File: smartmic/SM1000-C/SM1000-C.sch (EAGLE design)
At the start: 175 parts, among them CN1 HDR100-3, CN10 MJ-3523-SMT, CN11 HDR100-3, CN12 DF11-16DS, CN2 MOLEX-MINI-B-SMT, CN3 RASM712PX, CN4 RJ-45, CN5 MJ-3523-SMT, CN6 MJ-3523-SMT, CN7 MJ-3523-SMT, CN8 MJ-3523-SMT, CN9 MJ-3523-SMT, J1 JMP-2PIN, J3 JMP-2PIN, J4 JMP-2PIN, J5 JMP-2PIN, P1 TPAD50, P10 TPAD50, P11 TPAD50, P12 TPAD50, P13 TPAD50, P14 TPAD50, P15 TPAD50, P16 TPAD50, P17 TPAD50, P18 TPAD50, P19 TPAD50, P2 TPAD50, P20 TPAD50, P3 TPAD50, P4 TPAD50, P5 TPAD50, P6 TPAD50, P7 TPAD50, P8 TPAD50, P9 TPAD50, SW1 SW-BOURNS-7914S, SW2 SW-BOURNS-7914S, SW3 DPDT, SW4 SW-BOURNS-7914S, T1 SM-LP-5001, T2 SM-LP-5001, U1 STM32F405, U2 LD3985M33R, U3 STMPS2141, U4 EMIF02-USB03F2, U5 TPS54329E, U6 LMV341, U7 LMV341, U8 LM386M-1, U9 LMV341

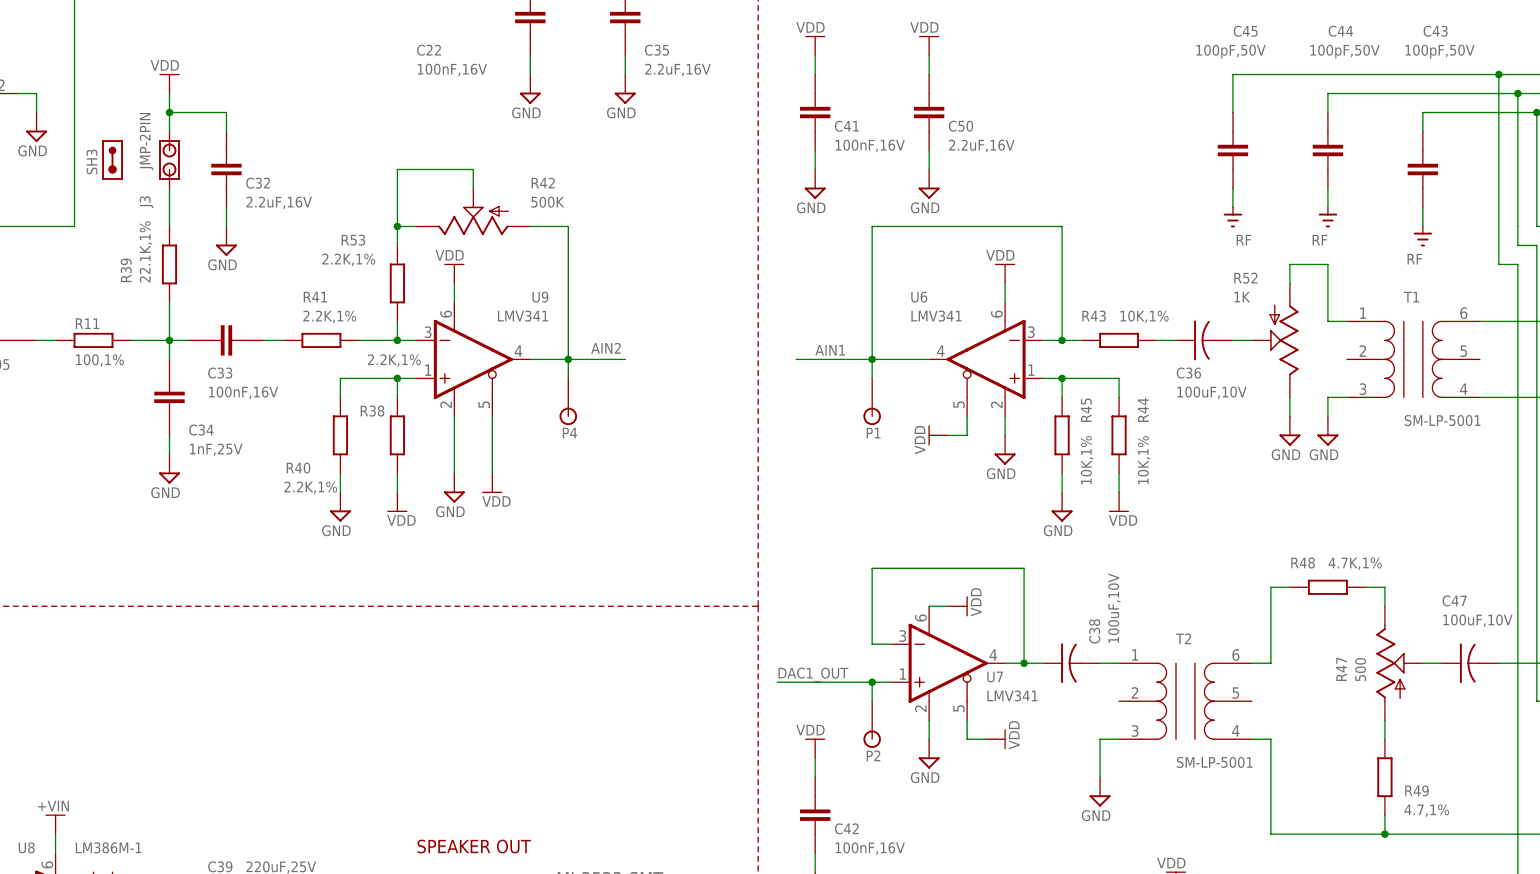
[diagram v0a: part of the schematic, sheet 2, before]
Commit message: Update to reflect review of Change-Log-C.txt  RGB 09/08/2014
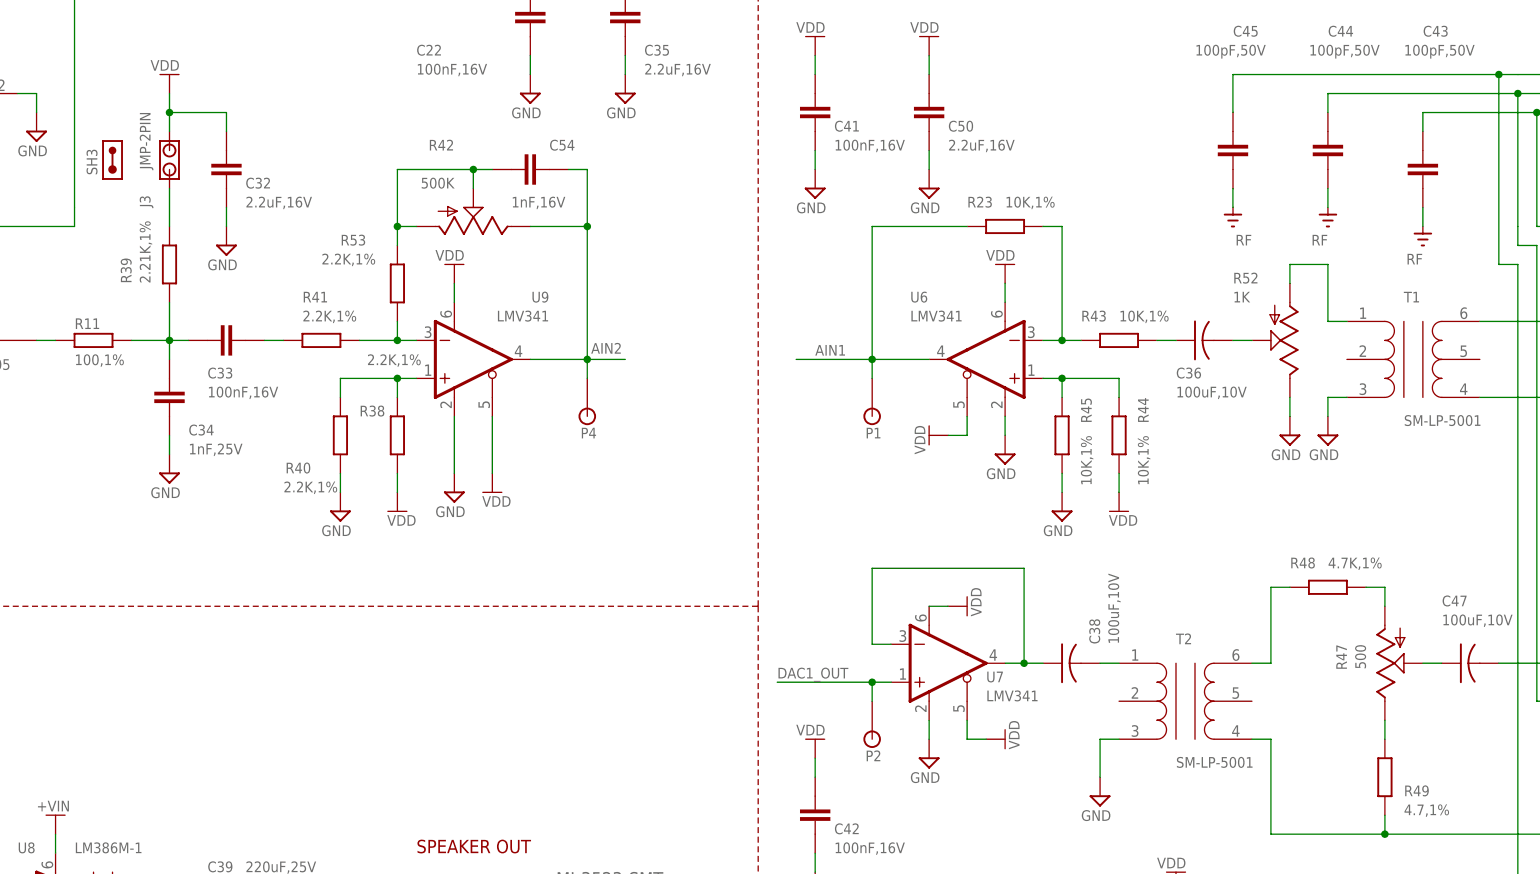
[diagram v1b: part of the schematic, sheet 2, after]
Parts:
- added C54: 1nF,16V, AA-ipc-7351-capacitor:CAPACITOR_0603
- added R23: 10K,1%, AA-ipc-7351-resistor:RESISTOR_0603
- R39: value 22.1K,1% -> 2.21K,1%
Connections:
- removed net N$81: R47.3, R49.2
- new net N$13: R47.1, R49.2
- new net N$14: R23.2, R43.1, U6.-IN
- net AIN1: now also R23.1; no longer R43.1, U6.-IN
- net AIN2: now also C54.2, R42.1; no longer R42.3
- net N$41: now also C54.1, R42.3; no longer R42.1
- net N$82: now also R47.3; no longer R47.1
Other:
- moved on the sheet: P4, R47
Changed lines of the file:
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@@
 <part name="V56" library="A-SUPPLY2" deviceset="GND" device=""/>
 <part name="C34" library="AA-ipc-7351-capacitor" deviceset="CAPACITOR_" device="0603" value="1nF,25V"/>
-<part name="R39" library="AA-ipc-7351-resistor" deviceset="RESISTOR_" device="0603" value="22.1K,1%"/>
+<part name="R39" library="AA-ipc-7351-resistor" deviceset="RESISTOR_" device="0603" value="2.21K,1%"/>
 <part name="R40" library="AA-ipc-7351-resistor" deviceset="RESISTOR_" device="0603" value="2.2K,1%"/>
 <part name="V59" library="A-SUPPLY2" deviceset="GND" device=""/>
@@
 <part name="R22" library="AA-ipc-7351-resistor" deviceset="RESISTOR_" device="0603" value="22.1K,1%"/>
 <part name="V125" library="A-SUPPLY2" deviceset="GND" device=""/>
+<part name="C54" library="AA-ipc-7351-capacitor" deviceset="CAPACITOR_" device="0603" value="1nF,16V"/>
+<part name="R23" library="AA-ipc-7351-resistor" deviceset="RESISTOR_" device="0603" value="10K,1%"/>
 </parts>
 <sheets>
@@
 </instance>
 <instance part="B-FRAME3" gate="G$3" x="355.6" y="279.4" smashed="yes"/>
-<instance part="R47" gate="G$1" x="238.76" y="88.9" smashed="yes">
-<attribute name="NAME" x="233.68" y="86.36" size="1.4224" layer="95" ratio="9" rot="R90"/>
-<attribute name="VALUE" x="236.22" y="86.36" size="1.4224" layer="96" ratio="9" rot="R90"/>
+<instance part="R47" gate="G$1" x="238.76" y="88.9" smashed="yes" rot="MR180">
+<attribute name="NAME" x="233.68" y="91.44" size="1.4224" layer="95" ratio="9" rot="MR270"/>
+<attribute name="VALUE" x="236.22" y="91.44" size="1.4224" layer="96" ratio="9" rot="MR270"/>
 </instance>
 <instance part="R52" gate="G$1" x="226.06" y="132.08" smashed="yes" rot="R180">
@@
 <attribute name="VALUE" x="93.98" y="134.62" size="1.4224" layer="96" ratio="9"/>
 </instance>
-<instance part="R42" gate="G$1" x="116.84" y="147.32" smashed="yes" rot="R90">
-<attribute name="NAME" x="124.46" y="152.4" size="1.4224" layer="95" ratio="9"/>
-<attribute name="VALUE" x="124.46" y="149.86" size="1.4224" layer="96" ratio="9"/>
+<instance part="R42" gate="G$1" x="116.84" y="147.32" smashed="yes" rot="MR90">
+<attribute name="NAME" x="114.3" y="157.48" size="1.4224" layer="95" ratio="9" rot="MR0"/>
+<attribute name="VALUE" x="114.3" y="152.4" size="1.4224" layer="96" ratio="9" rot="MR0"/>
 </instance>
 <instance part="V62" gate="GND" x="99.06" y="109.22" smashed="yes">
@@
 <instance part="P2" gate="G$1" x="170.18" y="83.82" rot="R180"/>
 <instance part="P3" gate="G$1" x="27.94" y="71.12"/>
-<instance part="P4" gate="G$1" x="129.54" y="127" rot="R180"/>
+<instance part="P4" gate="G$1" x="132.08" y="127" rot="R180"/>
 <instance part="C1" gate="G$1" x="101.6" y="251.46" smashed="yes" rot="R90">
 <attribute name="NAME" x="96.52" y="266.7" size="1.4224" layer="95"/>
@@
 <attribute name="VALUE" x="25.4" y="47.498" size="1.4224" layer="96" ratio="9"/>
 </instance>
+<instance part="C54" gate="G$1" x="124.46" y="154.94" smashed="yes">
+<attribute name="NAME" x="127" y="157.48" size="1.4224" layer="95"/>
+<attribute name="VALUE" x="121.92" y="149.86" size="1.4224" layer="96"/>
+</instance>
+<instance part="R23" gate="G$1" x="187.96" y="147.32" smashed="yes">
+<attribute name="NAME" x="182.88" y="149.86" size="1.4224" layer="95" ratio="9"/>
+<attribute name="VALUE" x="187.96" y="149.86" size="1.4224" layer="96" ratio="9"/>
+</instance>
 </instances>
 <busses>
@@
 <segment>
 <label x="132.588" y="130.302" size="1.4224" layer="95" ratio="10"/>
-<wire x1="129.54" y1="129.54" x2="137.16" y2="129.54" width="0.1524" layer="91"/>
+<wire x1="132.08" y1="129.54" x2="137.16" y2="129.54" width="0.1524" layer="91"/>
 <pinref part="U9" gate="G$1" pin="OUT"/>
-<wire x1="124.46" y1="129.54" x2="129.54" y2="129.54" width="0.1524" layer="91"/>
-<pinref part="R42" gate="G$1" pin="3"/>
-<wire x1="124.46" y1="147.32" x2="129.54" y2="147.32" width="0.1524" layer="91"/>
-<wire x1="129.54" y1="147.32" x2="129.54" y2="129.54" width="0.1524" layer="91"/>
-<wire x1="129.54" y1="127" x2="129.54" y2="129.54" width="0.1524" layer="91"/>
+<wire x1="124.46" y1="129.54" x2="132.08" y2="129.54" width="0.1524" layer="91"/>
+<wire x1="132.08" y1="147.32" x2="132.08" y2="129.54" width="0.1524" layer="91"/>
+<wire x1="132.08" y1="127" x2="132.08" y2="129.54" width="0.1524" layer="91"/>
 <pinref part="P4" gate="G$1" pin="1"/>
-<junction x="129.54" y="129.54"/>
+<junction x="132.08" y="129.54"/>
+<pinref part="C54" gate="G$1" pin="2"/>
+<wire x1="129.54" y1="154.94" x2="132.08" y2="154.94" width="0.1524" layer="91"/>
+<wire x1="132.08" y1="154.94" x2="132.08" y2="147.32" width="0.1524" layer="91"/>
+<pinref part="R42" gate="G$1" pin="1"/>
+<wire x1="124.46" y1="147.32" x2="132.08" y2="147.32" width="0.1524" layer="91"/>
+<junction x="132.08" y="147.32"/>
 </segment>
 </net>
@@
 <wire x1="177.8" y1="129.54" x2="170.18" y2="129.54" width="0.1524" layer="91"/>
 <wire x1="170.18" y1="127" x2="170.18" y2="129.54" width="0.1524" layer="91"/>
-<pinref part="U6" gate="G$1" pin="-IN"/>
-<wire x1="193.04" y1="132.08" x2="195.58" y2="132.08" width="0.1524" layer="91"/>
-<pinref part="R43" gate="G$1" pin="1"/>
-<wire x1="195.58" y1="132.08" x2="198.12" y2="132.08" width="0.1524" layer="91"/>
-<wire x1="195.58" y1="132.08" x2="195.58" y2="147.32" width="0.1524" layer="91"/>
-<wire x1="195.58" y1="147.32" x2="170.18" y2="147.32" width="0.1524" layer="91"/>
-<junction x="195.58" y="132.08"/>
 <wire x1="170.18" y1="129.54" x2="170.18" y2="147.32" width="0.1524" layer="91"/>
 <pinref part="P1" gate="G$1" pin="1"/>
 <junction x="170.18" y="129.54"/>
+<pinref part="R23" gate="G$1" pin="1"/>
+<wire x1="170.18" y1="147.32" x2="182.88" y2="147.32" width="0.1524" layer="91"/>
 </segment>
 </net>
@@
 </segment>
 </net>
-<net name="N$81" class="0">
-<segment>
-<pinref part="R49" gate="G$1" pin="2"/>
-<pinref part="R47" gate="G$1" pin="3"/>
-<wire x1="238.76" y1="78.74" x2="238.76" y2="81.28" width="0.1524" layer="91"/>
-</segment>
-</net>
 <net name="N$82" class="0">
 <segment>
-<pinref part="R47" gate="G$1" pin="1"/>
-<wire x1="238.76" y1="96.52" x2="238.76" y2="99.06" width="0.1524" layer="91"/>
 <pinref part="R48" gate="G$1" pin="1"/>
 <wire x1="238.76" y1="99.06" x2="236.22" y2="99.06" width="0.1524" layer="91"/>
+<pinref part="R47" gate="G$1" pin="3"/>
+<wire x1="238.76" y1="96.52" x2="238.76" y2="99.06" width="0.1524" layer="91"/>
 </segment>
 </net>
@@
 </segment>
 </net>
-<net name="N$61" class="0">
-<segment>
-<pinref part="R47" gate="G$1" pin="2"/>
-<pinref part="C47" gate="G$1" pin="1"/>
-<wire x1="243.84" y1="88.9" x2="246.38" y2="88.9" width="0.1524" layer="91"/>
-</segment>
-</net>
 <net name="N$79" class="0">
 <segment>
@@
 <net name="N$41" class="0">
 <segment>
-<wire x1="106.68" y1="147.32" x2="109.22" y2="147.32" width="0.1524" layer="91"/>
-<pinref part="R42" gate="G$1" pin="1"/>
-<pinref part="R42" gate="G$1" pin="2"/>
-<wire x1="116.84" y1="152.4" x2="116.84" y2="154.94" width="0.1524" layer="91"/>
 <wire x1="116.84" y1="154.94" x2="106.68" y2="154.94" width="0.1524" layer="91"/>
 <wire x1="106.68" y1="154.94" x2="106.68" y2="147.32" width="0.1524" layer="91"/>
 <pinref part="R53" gate="G$1" pin="2"/>
 <wire x1="106.68" y1="144.78" x2="106.68" y2="147.32" width="0.1524" layer="91"/>
+<pinref part="C54" gate="G$1" pin="1"/>
+<wire x1="116.84" y1="154.94" x2="119.38" y2="154.94" width="0.1524" layer="91"/>
+<pinref part="R42" gate="G$1" pin="2"/>
+<wire x1="116.84" y1="152.4" x2="116.84" y2="154.94" width="0.1524" layer="91"/>
+<pinref part="R42" gate="G$1" pin="3"/>
+<wire x1="109.22" y1="147.32" x2="106.68" y2="147.32" width="0.1524" layer="91"/>
 <junction x="106.68" y="147.32"/>
+<junction x="116.84" y="154.94"/>
 </segment>
 </net>
@@
 </segment>
 </net>
+<net name="N$11" class="0">
+<segment>
+<pinref part="R47" gate="G$1" pin="2"/>
+<pinref part="C47" gate="G$1" pin="1"/>
+<wire x1="243.84" y1="88.9" x2="246.38" y2="88.9" width="0.1524" layer="91"/>
+</segment>
+</net>
+<net name="N$13" class="0">
+<segment>
+<pinref part="R47" gate="G$1" pin="1"/>
+<pinref part="R49" gate="G$1" pin="2"/>
+<wire x1="238.76" y1="81.28" x2="238.76" y2="78.74" width="0.1524" layer="91"/>
+</segment>
+</net>
+<net name="N$14" class="0">
+<segment>
+<pinref part="R43" gate="G$1" pin="1"/>
+<wire x1="195.58" y1="132.08" x2="198.12" y2="132.08" width="0.1524" layer="91"/>
+<wire x1="195.58" y1="132.08" x2="195.58" y2="147.32" width="0.1524" layer="91"/>
+<junction x="195.58" y="132.08"/>
+<pinref part="U6" gate="G$1" pin="-IN"/>
+<wire x1="193.04" y1="132.08" x2="195.58" y2="132.08" width="0.1524" layer="91"/>
+<pinref part="R23" gate="G$1" pin="2"/>
+<wire x1="193.04" y1="147.32" x2="195.58" y2="147.32" width="0.1524" layer="91"/>
+</segment>
+</net>
